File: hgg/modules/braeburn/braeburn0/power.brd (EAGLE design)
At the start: 100.5 x 80 mm, 54 parts, among them IC1 7812TV, IC2 7805TV, IC3 7805TV, IC4 ATMEGA48/88/168-AU

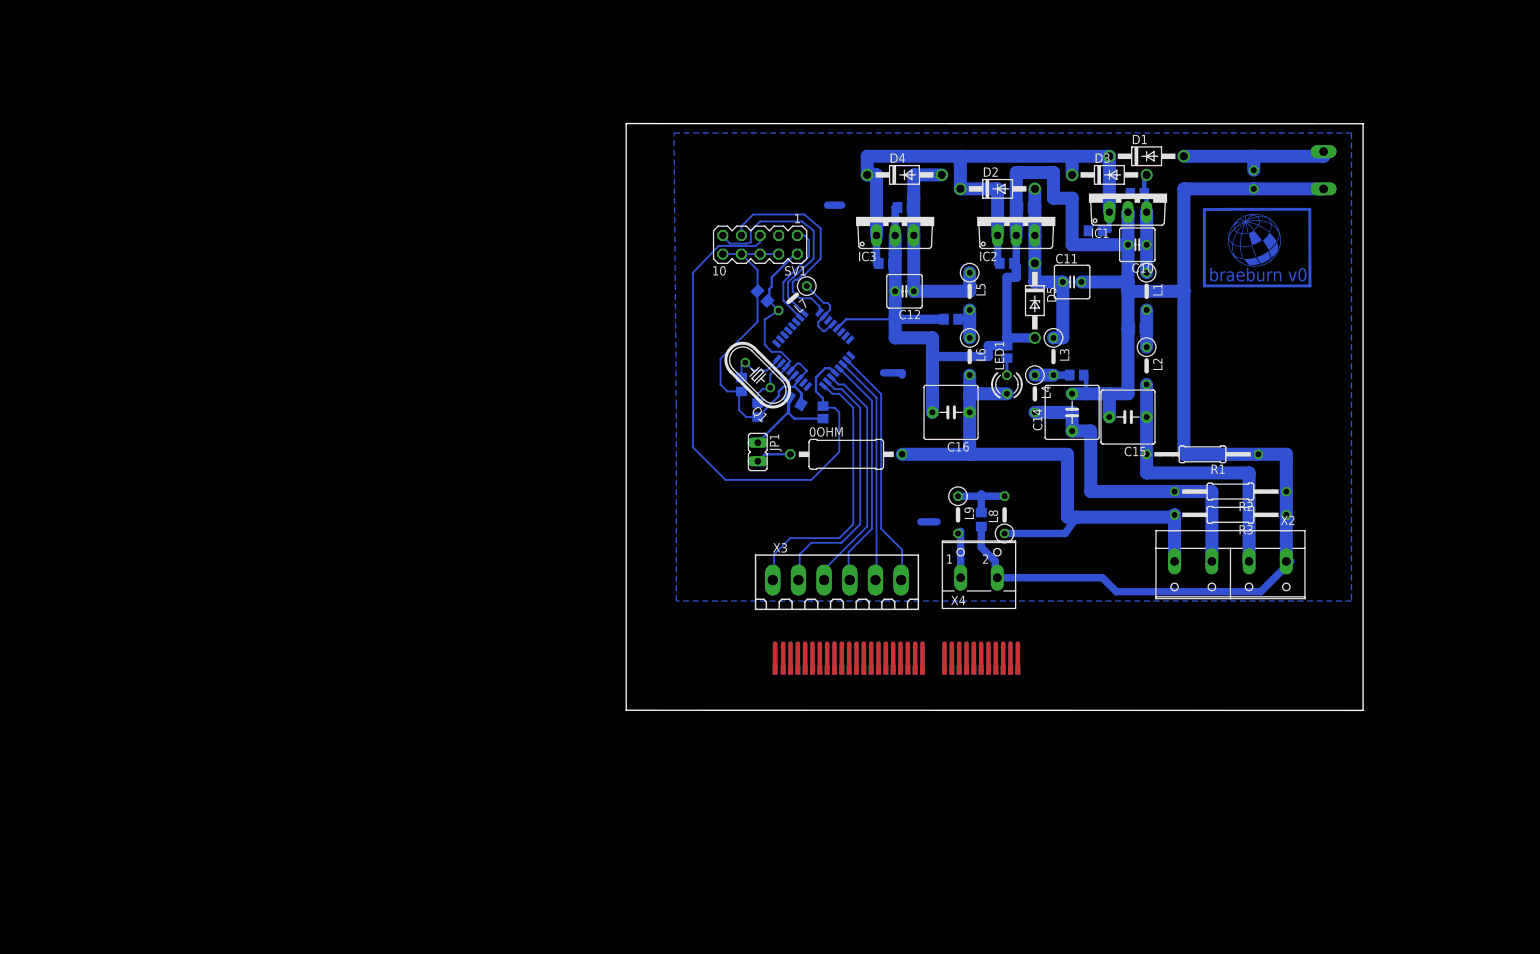
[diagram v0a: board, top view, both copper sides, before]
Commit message: new release of braeburn board file
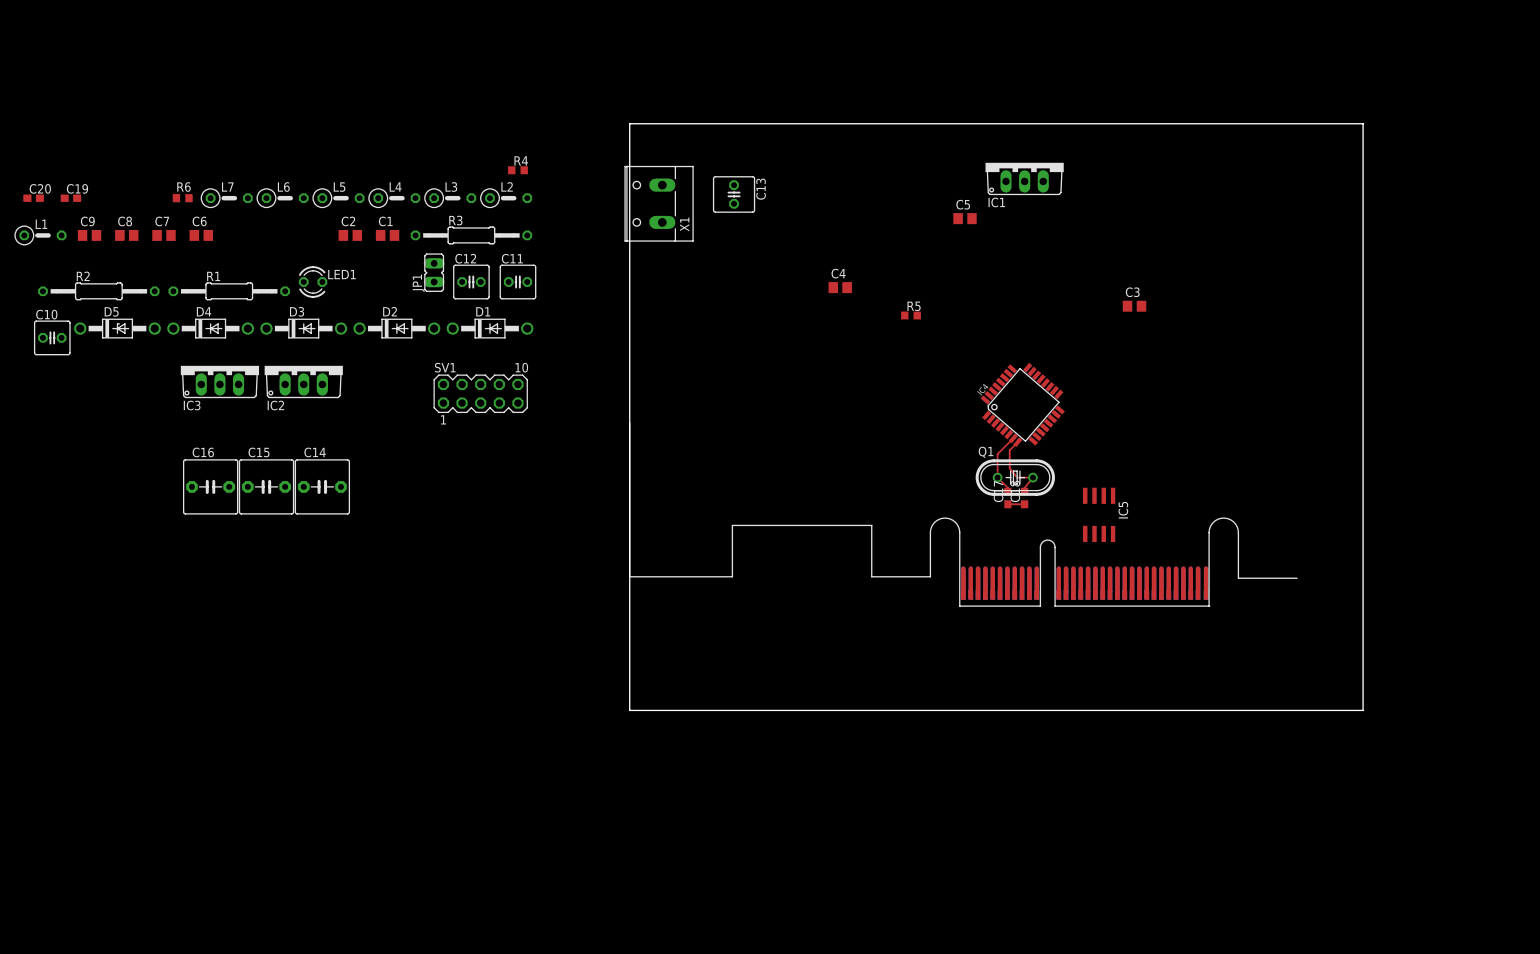
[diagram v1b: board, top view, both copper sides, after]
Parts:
- removed 0OHM: (no value), rcl:0411/15
- removed C21: (no value), rcl:C0805
- removed L8, L9: (no value), rcl:0207/5V
- removed X2: (no value), con-wago-508:W237-4P
- removed X3: (no value), con-weidmueller-sl35:180G-6
- removed X4: (no value), con-wago-500:W237-102
- added IC5: LTC485S, linear-technology:SOIC8
- added R5: 30K, rcl:R0603
- C17, C18, C19, C20: device rcl:C0805 -> rcl:C0603
- R4: device rcl:R2012 -> rcl:R0603
- R6: device resistor:R0805 -> resistor:R0603
- U$1: value FRIENDSHIPEDGECONNECTOR -> FRIENDSHIPCONNECTOR
- moved R2 156.7 mm to (-72.4, 57.1), turned to 0 degrees
- moved L1 150.7 mm to (-80.0, 64.8), turned to 0 degrees
- moved C10 148.5 mm to (-78.7, 50.8), turned to 0 degrees
- moved R1 134.6 mm to (-54.6, 57.1), turned to 0 degrees
- moved D5 125.2 mm to (-69.8, 52.1), turned to 0 degrees
- moved C9 118.0 mm to (-73.7, 64.8), flipped to the top
- moved C15 117.9 mm to (-49.5, 30.5), turned to 0 degrees
- moved D3 111.8 mm to (-44.5, 52.1)
- moved R3 110.3 mm to (-21.6, 64.8), turned to 0 degrees
- moved C6 109.9 mm to (-58.4, 64.8), flipped to the top, turned to 0 degrees
- moved C2 107.5 mm to (-38.1, 64.8), flipped to the top
- moved C20 107.4 mm to (-81.3, 69.8), flipped to the top, turned to 0 degrees
- moved C8 106.1 mm to (-68.6, 64.8), flipped to the top
- moved C14 102.7 mm to (-41.9, 30.5), turned to 0 degrees
- moved C16 101.5 mm to (-57.1, 30.5), turned to 0 degrees
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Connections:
- new net N$31: C16.1, JP1.1, L6.2, R3.2, U$1.A08(+5V), U$1.B08(+5V)
- new net N$32: IC4.25, IC5.2, IC5.3, R5.2
- new net N$33: IC4.1, U$1.A03(/CS,IRQ)
- new net N$34: IC4.2, U$1.A02(IRQ)
- net GND: now also IC5.5, U$1.A07(GND), U$1.A09(GND), U$1.A11(GND), U$1.A19(GND), U$1.B07(GND), U$1.B09(GND), U$1.B11(GND); no longer C21.1, X2.1, X4.2
- net N$10: now also IC5.8, R5.1, U$1.A06(+3V3), U$1.B06(+3V3); no longer X2.3
- net N$11: now also IC5.6, U$1.A17(BUS0-); no longer 0OHM.2, C16.1, L6.2, L8.1, LED1.A, R3.2, X2.4
- net N$20: now also U$1.A26(PPS); no longer X3.1
- net N$21: now also IC5.4; no longer X3.2
- net N$22: now also IC5.7, U$1.A18(BUS0+); no longer IC4.30, X3.3
- net N$23: now also U$1.A01(PRSNT1), U$1.A32(PRSNT2); no longer IC4.28, X3.4
- net N$24: now also U$1.A24(SLOWCLKCLK); no longer X3.5
- net N$25: now also U$1.A23(SLOWTIMEMOSI); no longer X3.6
- net N$27: no longer JP1.1
- net N$28: now also U$1.A10(+12V), U$1.B10(+12V); no longer X2.2
- net N$29: now also U$1.A12(TDI), U$1.A13(TDO); no longer C21.2, L8.2, L9.1
- net N$30: now also IC4.30, IC5.1; no longer L9.2, X4.1
- net N$9: now also LED1.A; no longer 0OHM.1
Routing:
- net GND: track 375.4 -> 2.29 mm
- net N$1: track 82.9 -> 0.00 mm
- net N$11: track 79.2 -> 0.00 mm
- net N$14: track 74.7 -> 0.00 mm
- net N$26: track 49.6 -> 0.00 mm
- net N$10: track 44.5 -> 0.00 mm
- net N$27: track 43.0 -> 0.00 mm
- net N$28: track 38.1 -> 0.00 mm
- net N$20: track 37.3 -> 0.00 mm
- net N$21: track 35.4 -> 0.00 mm
- net N$25: track 33.2 -> 0.00 mm
- net N$22: track 32.7 -> 0.00 mm
- net N$23: track 32.1 -> 0.00 mm
- net N$24: track 31.4 -> 0.00 mm
- net N$3: track 31.2 -> 0.00 mm
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- removed copper zone on layer 16, net GND
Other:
- board size 100.5 x 80 mm -> 100 x 80 mm
- board text removed: "braeburn v0"

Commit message: initial version of design update
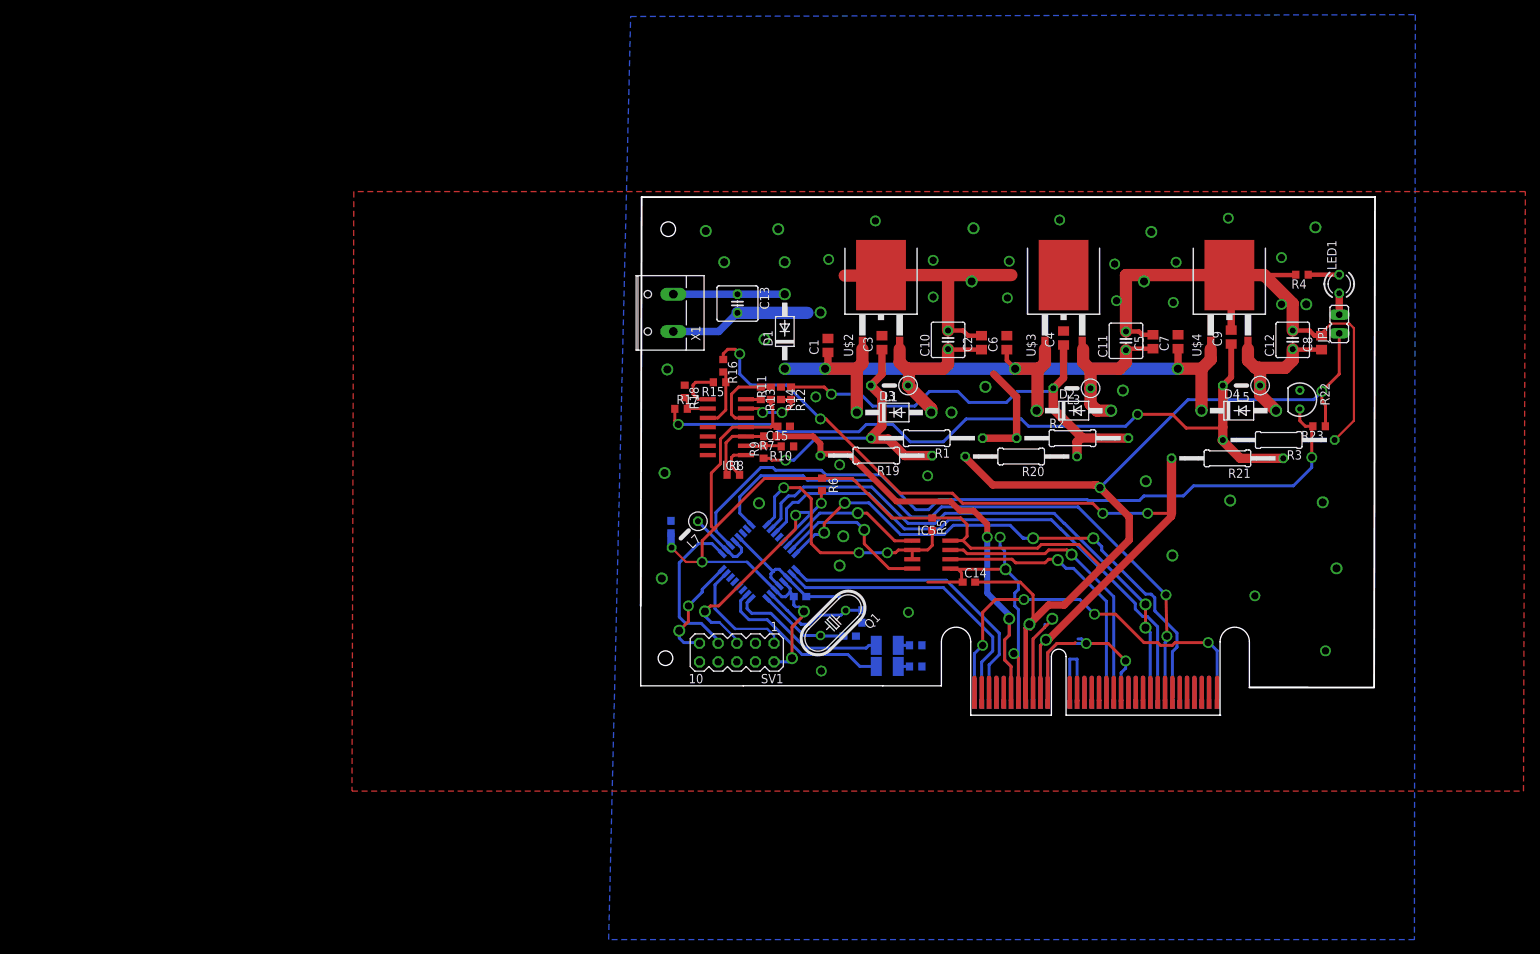
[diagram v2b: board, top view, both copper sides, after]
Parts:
- removed C16: (no value), capacitor-wima:C5B7.2
- removed D5: 1N4728, diode:DO41Z10
- removed IC2, IC3: 7805TV, linear:TO220V
- removed L2, L4, L6: (no value), resistor:0207/5V
- added LED2, LED4: GM5BW96385A, led:GM5BW96385A
- added R10, R11, R12, R13, R14, R15, R16, R17, R18, R7, R8, R9: (no value), rcl:R0603
- added R19, R20, R21: (no value), rcl:0207/15
- added R22: PTC-SOD70, ptc-ntc:SOD70
- added R23, R24, R25: 2k, rcl:R0603
- added U$2, U$3, U$4: AP1084, hgg:TO263
- C13: value (none) -> 2000u
- C14: value (none) -> 100n; device capacitor-wima:C5B7.2 -> rcl:C0603
- C15: device capacitor-wima:C5B7.2 -> rcl:C0603
- C17, C18: value (none) -> 22n
- C19: value (none) -> 2n2
- C20: value (none) -> 100n
- IC1: value 7812TV -> LM324D; device linear:TO220V -> linear:SO14
- L7: value (none) -> 33u
- R5: value 30K -> 10k
- R6: value (none) -> 10k
- moved C8 163.6 mm to (94.3, 50.1), turned to 90 degrees
- moved C9 156.3 mm to (82.0, 50.9), turned to 90 degrees
- moved D4 140.6 mm to (83.0, 40.9)
- moved LED1 139.9 mm to (96.8, 58.1), turned to 90 degrees
- moved C7 139.0 mm to (74.8, 50.3), turned to 90 degrees
- moved R2 134.3 mm to (60.4, 37.1)
- moved L5 125.4 mm to (83.4, 44.3), turned to 180 degrees
- moved JP1 123.6 mm to (96.8, 52.7)
- moved C10 122.2 mm to (43.4, 50.5), turned to 90 degrees
- moved C20 117.8 mm to (23.2, 15.5), flipped to the bottom, turned to 180 degrees
- moved L1 117.2 mm to (35.4, 44.3), turned to 180 degrees
- moved R3 113.6 mm to (88.5, 36.9), turned to 180 degrees
- moved C12 112.3 mm to (90.4, 50.5), turned to 90 degrees
- moved C6 110.8 mm to (51.4, 50.1), turned to 90 degrees
- moved R4 107.9 mm to (91.7, 59.4), turned to 180 degrees
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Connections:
- net N$11 renamed BUS0-
- net N$14 renamed RST
- net N$22 renamed BUS0+
- net N$33 renamed /CS
- net N$34 renamed IRQ
- removed net N$31: C16.1, JP1.1, L6.2, R3.2, U$1.A08(+5V), U$1.B08(+5V)
- new net 12V: R16.1, R21.2, U$1.A10(+12V), U$1.B10(+12V)
- new net 12VIN: C9.1, L5.2, R17.1, R21.1, R3.2
- new net 3V3: R19.2, R7.1, U$1.A06(+3V3), U$1.B06(+3V3)
- new net 3V3IN: C3.1, L1.2, R1.2, R19.1, R9.1
- new net LED1: IC4.9, LED2.A
- new net LED2: IC4.10, LED4.A
- new net N$11: IC1.7, R13.2
- new net N$14: IC1.6, R12.2, R14.2
- new net N$22: IC1.5, R11.2, R13.1
- new net N$26: IC1.10, R15.1, R16.2
- new net N$36: LED2.C, R24.1
- new net N$37: LED4.C, R25.1
- new net TEMP1: IC4.19, R22.2, R23.2
- new net VCC: C14.2, C15.2, C19.1, C20.1, IC1.4, IC4.4, IC4.6, IC5.8, JP1.1, L7.2, R11.1, R20.2, R23.1, R5.1, R6.1, SV1.2, U$1.A08(+5V), U$1.B08(+5V)
- new net VCCIN: C4.1, L3.2, R12.1, R2.2, R20.1
- net GND: now also C14.1, C15.1, IC1.11, R10.1, R14.1, R18.1, R22.1, R24.2, R25.2, U$2.3, U$3.3, U$4.3; no longer C14.2, C15.2, C16.2, D5.A, IC1.2, IC2.2, IC3.2
- net N$1: now also U$2.1, U$3.1, U$4.1; no longer IC1.1, IC2.1, IC3.1
- net N$10: now also IC1.1, R8.2; no longer C14.1, IC5.8, L4.2, R2.2, R5.1, U$1.A06(+3V3), U$1.B06(+3V3)
- net N$27: now also IC1.8, R15.2; no longer C19.1, C20.1, IC4.4, IC4.6, L7.2, R6.1, SV1.2
- net N$28: now also IC1.9, R17.2, R18.2; no longer C15.1, L2.2, R1.2, U$1.A10(+12V), U$1.B10(+12V)
- net N$3: now also U$4.2; no longer IC3.3
- net N$4: now also U$3.2; no longer D5.C, IC2.3
- net N$5: now also U$2.2; no longer IC1.3
- net N$6: now also IC4.24, U$1.A25(SLOWCLK/CS); no longer C9.1, L5.2, L6.1
- net N$7: now also IC1.2, R10.2, R9.2; no longer C4.1, L3.2, L4.1
- net N$8: now also IC1.3, R7.2, R8.1; no longer C3.1, L1.2, L2.1
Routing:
- net GND: track 2.29 -> 282.3 mm, vias 0 -> 53
- net VCC: track 0.00 -> 267.1 mm, vias 0 -> 6
- net 12V: track 0.00 -> 123.4 mm, vias 0 -> 5
- net 12VIN: track 0.00 -> 104.6 mm, vias 0 -> 2
- net TEMP1: track 0.00 -> 103.5 mm, vias 0 -> 1
- net N$1: track 0.00 -> 100.0 mm, vias 0 -> 3
- net N$6: track 0.00 -> 86.6 mm, vias 0 -> 2
- net N$25: track 0.00 -> 76.4 mm, vias 0 -> 2
- net N$20: track 0.00 -> 75.4 mm, vias 0 -> 4
- net N$24: track 0.00 -> 75.0 mm
- net 3V3: track 0.00 -> 73.8 mm, vias 0 -> 2
- net VCCIN: track 0.00 -> 63.2 mm, vias 0 -> 1
- net N$23: track 0.00 -> 56.2 mm, vias 0 -> 4
- net /CS: track 0.00 -> 41.6 mm
- net IRQ: track 0.00 -> 40.8 mm
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- added copper zone on layer 1, net GND
- added copper zone on layer 16, net GND
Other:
- board size 100 x 80 mm -> 100.1 x 66.9 mm
